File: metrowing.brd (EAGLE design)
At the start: 68.6 x 53.5 mm, 8 parts, among them SW1 SPST_TACT-KMR2, U2 ARDUINOR3-NOSILK

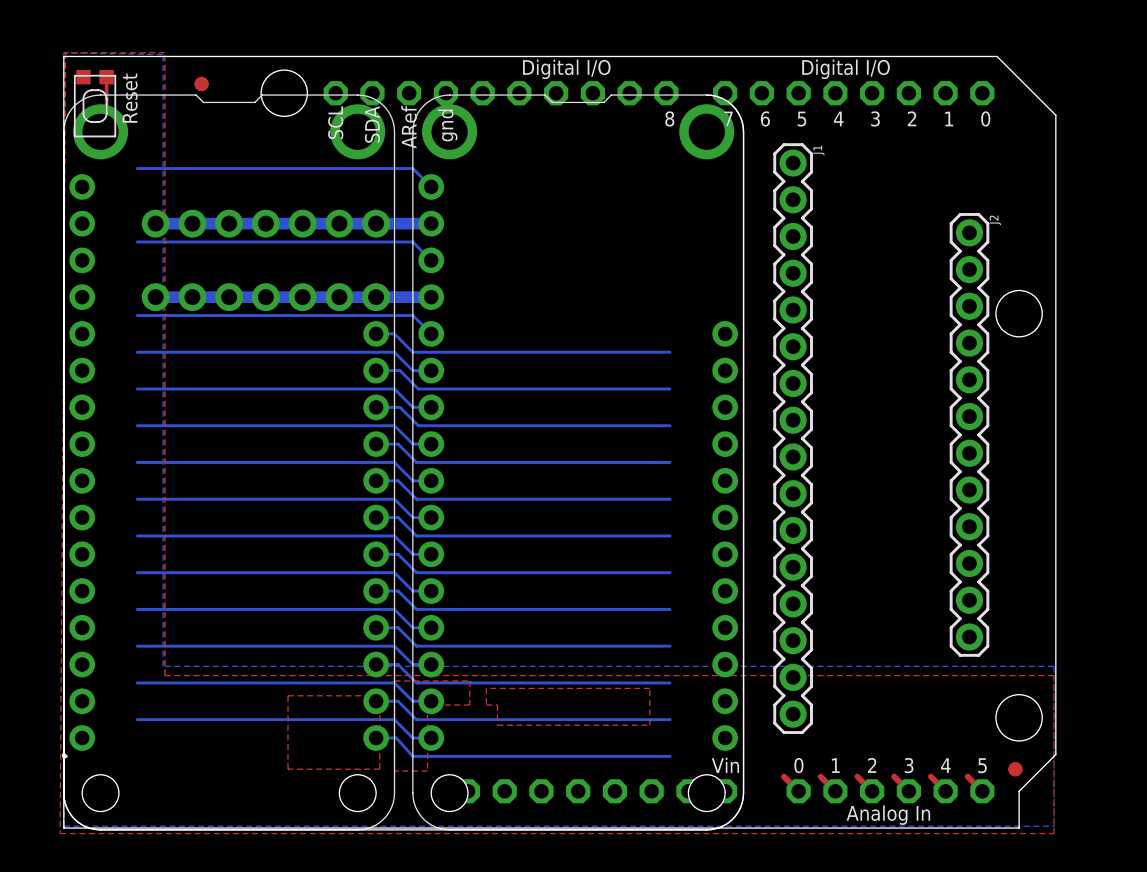
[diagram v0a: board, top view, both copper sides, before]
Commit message: correct (mkii) version
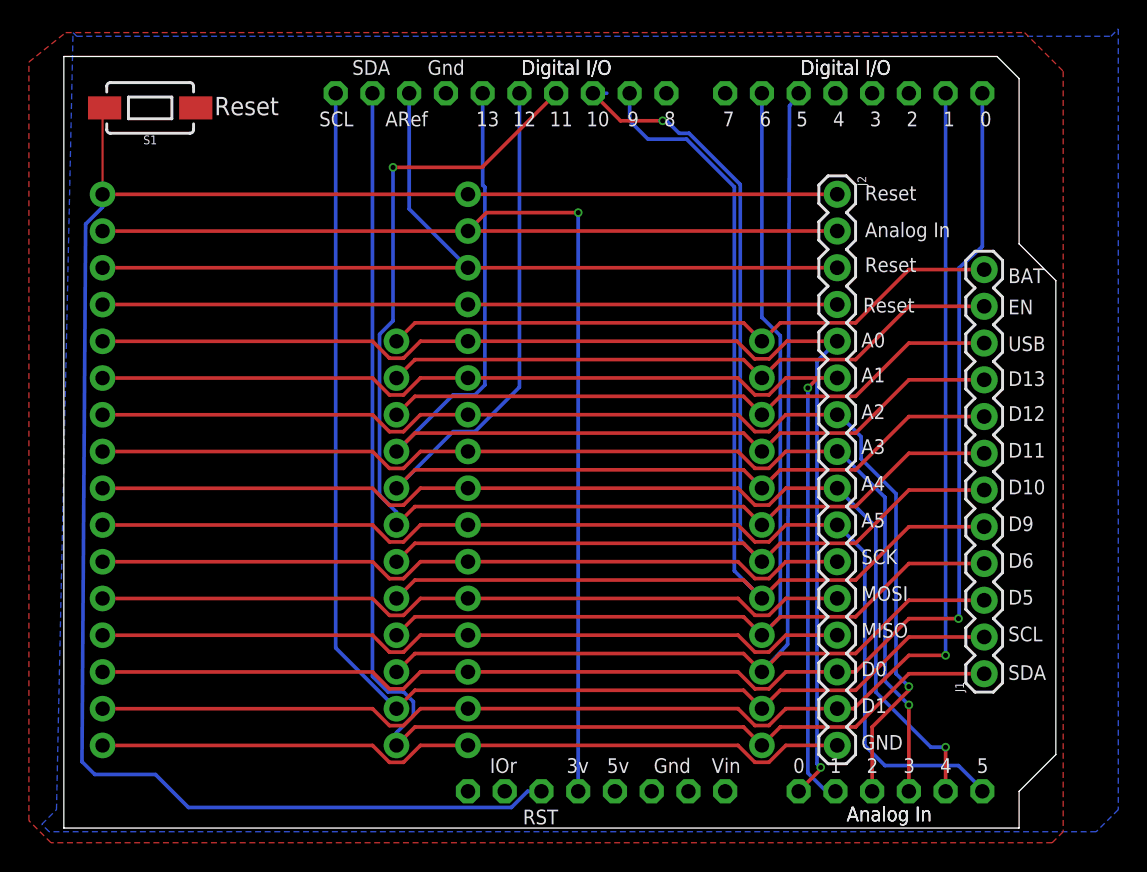
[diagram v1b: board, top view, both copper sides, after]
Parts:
- removed SW1: SPST_TACT-KMR2, adafruit:KMR2
- removed U$3, U$4: FIDUCIAL, adafruit:FIDUCIAL_1MM
- removed U2: ARDUINOR3-NOSILK, microbuilder:ARDUINOR3-NOSILK
- added S1: MOMENTARY-SWITCH-SPST-SMD-6.0X3.5MM, SparkFun-Switches:TACTILE_SWITCH_SMD_6.0X3.5MM
- added U1: ARDUINOR3-DIMENSION, 00_bsiepert:ARDUINOR3
- J1: device SparkFun-Connectors:1X16 -> SparkFun-Connectors:1X12
- J2: device SparkFun-Connectors:1X12 -> SparkFun-Connectors:1X16
- MS1, MS2: value FEATHERWING_NODIM -> FEATHERWING_PINS; device microbuilder:FEATHERWING_DIM -> 00_bsiepert:FEATHERWING_PINS
- moved J1 37.7 mm to (63.6, 10.7), turned to 90 degrees
- moved J2 9.52 mm to (53.5, 43.8)
- moved MS2 2.59 mm to (26.7, 50.2)
- moved MS1 1.50 mm to (1.41, 50.2)
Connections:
- removed net 3V: J1.2, MS1.2, MS2.2, U2.3V
- removed net N$5: J2.2, MS1.27, MS2.27
- removed net RST: J1.1, MS1.1, MS2.1
- removed net VIN: U2.VIN
- new net 3V3: J2.2, MS1.2, MS2.2, U1.3V
- new net D2: U1.D2
- new net D3: U1.D3
- new net D4: U1.D4
- new net D7: U1.D7
- new net D8: U1.D8
- new net ENABLE: J1.11, MS1.27, MS2.27
- new net IOREF: U1.IOREF
- new net N$153: U1.VIN
- new net N$4: U1.RESERVED
- net +5V: now also U1.5V; no longer U2.5V
- net A0: now also J2.5, U1.A0; no longer J1.5, U2.A0
- net A1: now also J2.6, U1.A1; no longer J1.6, U2.A1
- net A2: now also J2.7, U1.A2; no longer J1.7, U2.A2
- net A3: now also J2.8, U1.A3; no longer J1.8, U2.A3
- net A4: now also J2.9, U1.A4; no longer J1.9, U2.A4
- net A5: now also J2.10, U1.A5; no longer J1.10, U2.A5
- net AREF: now also J2.3, U1.AREF; no longer J1.3, U2.AREF
- net D0: now also J2.14, U1.D0; no longer J1.14, U2.D0
- net D1: now also J2.15, U1.D1; no longer J1.15, U2.D1
- net D10: now also J1.6, U1.D10; no longer J2.7
- net D11: now also J1.7, U1.D11; no longer J2.6
- net D12: now also J1.8, U1.D12; no longer J2.5
- net D13: now also J1.9, U1.D13; no longer J2.4
- net D5: now also J1.3, U1.D5; no longer J2.10
- net D6: now also J1.4, U1.D6; no longer J2.9
- net D9: now also J1.5, U1.D9; no longer J2.8
- net GND: now also J2.16, J2.4, S1.1, U1.GND, U1.GND1, U1.GND2; no longer J1.16, J1.4, SW1.1, SW1.3, U2.GND, U2.GND1, U2.GND2
- net MISO: now also J2.13; no longer J1.13
- net MOSI: now also J2.12; no longer J1.12
- net RESET: now also J2.1, MS1.1, MS2.1, S1.2, U1.RESET; no longer SW1.2, SW1.4, U2.RESET
- net SCK: now also J2.11; no longer J1.11
- net SCL: now also J1.2, U1.SCL; no longer J2.11, U2.SCL
- net SDA: now also J1.1, U1.SDA; no longer J2.12, U2.SDA
- net USB: now also J1.10; no longer J2.3
- net VBAT: now also J1.12; no longer J2.1
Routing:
- net RESET: track 4.00 -> 130.1 mm
- net 3V3: track 0.00 -> 98.9 mm, vias 0 -> 1
- net D1: track 20.8 -> 100.6 mm, vias 0 -> 1
- net D0: track 20.8 -> 99.7 mm, vias 0 -> 1
- net SDA: track 20.9 -> 91.1 mm
- net SCL: track 20.8 -> 88.0 mm
- net GND: track 39.9 -> 103.5 mm, vias 7 -> 0
- net D10: track 20.8 -> 84.2 mm, vias 0 -> 1
- net D5: track 21.4 -> 84.6 mm
- net D9: track 20.8 -> 84.0 mm
- net A0: track 22.3 -> 85.2 mm, vias 0 -> 1
- net D11: track 20.8 -> 82.7 mm, vias 0 -> 1
- net D6: track 20.8 -> 82.3 mm
- net A1: track 22.3 -> 82.7 mm, vias 0 -> 1
- net A2: track 22.3 -> 81.9 mm, vias 0 -> 1
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- removed copper zone on layer 1, net N$4
- removed copper zone on layer 1, net VBAT
- removed copper zone on layer 1, net VOUT
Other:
- board size 68.6 x 53.5 mm -> 68.6 x 53.3 mm
- board text added: "A0"
- board text added: "A1"
- board text added: "A2"
- board text added: "A3"
- board text added: "A4"
- board text added: "A5"
- board text added: "BAT"
- board text added: "D0"
- board text added: "D1"
- board text added: "D10"
- board text added: "D11"
- board text added: "D12"
- board text added: "D13"
- board text added: "D5"
- board text added: "D6"
- board text added: "D9"
- board text added: "EN"
- board text added: "GND"
- board text added: "MISO"
- board text added: "MOSI"
- board text added: "SCK"
- board text added: "USB"
- board text removed: "0"
- board text removed: "1"
- board text removed: "2"
- board text removed: "3"
- board text removed: "4"
- board text removed: "5"
- board text removed: "6"
- board text removed: "7"
- board text removed: "8"
- board text removed: "ARef"
- board text removed: "Vin"
- board text removed: "gnd"
